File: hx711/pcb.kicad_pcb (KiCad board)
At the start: 4 copper layers, 70 x 22 mm, 65 parts, among them J1 RJ45_LED, J2 CONN_01X05, J3 CONN_01X05, J4 CONN_01X05, J5 CONN_01X05, U1 sp485, U10 CMC, U11 CMC, U12 CMC, U13 CMC, U14 CMC, U2 sp485, U3 sp485, U4 20M, U5 LDO, U6 USBLC6-4SC6, U7 USBLC6-4SC6, U8 HX711, U9 HX711

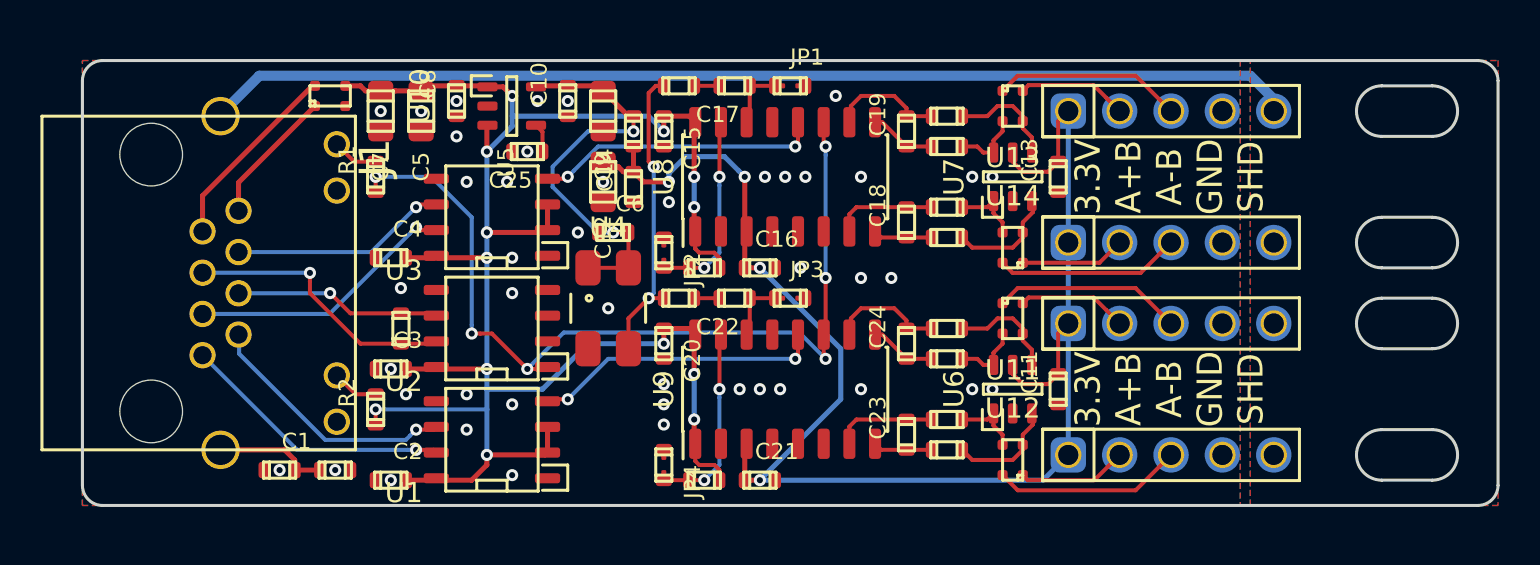
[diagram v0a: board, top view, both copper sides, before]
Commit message: jlc export
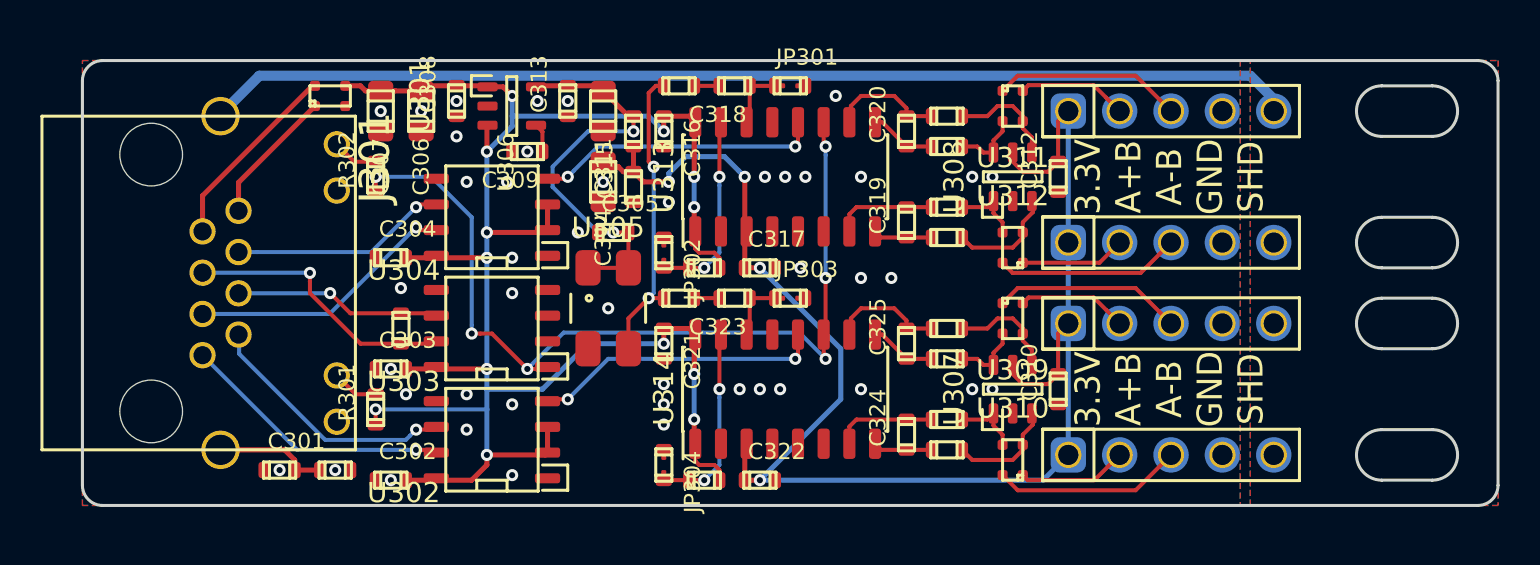
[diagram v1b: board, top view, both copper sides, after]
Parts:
- renumbered C1 to C301, C2 to C302, C3 to C303, C4 to C304, C6 to C305, C5 to C306, C7 to C307, C8 to C308, C25 to C309, C11 to C310, C9 to C311, C13 to C312, C10 to C313, C12 to C314, C14 to C315, C15 to C316, C16 to C317, C17 to C318, C18 to C319, C19 to C320, C20 to C321, C21 to C322, C22 to C323, C23 to C324, C24 to C325, J1 to J301, J2 to J302, J3 to J303, J4 to J304, J5 to J305, JP1 to JP301, JP2 to JP302, JP3 to JP303, JP4 to JP304, L1 to L301, R2 to R301, R1 to R302, R3 to R303, R16 to R304, R4 to R305, R5 to R306, R6 to R307, R7 to R308, R8 to R309, R9 to R310, R10 to R311, R11 to R312, R12 to R313, R13 to R314, R14 to R315, R15 to R316, U10 to U301, U1 to U302, U2 to U303, U3 to U304, U4 to U305, U5 to U306, U6 to U307, U7 to U308, U11 to U309, U12 to U310, U13 to U311, U14 to U312, U8 to U313, U9 to U314
